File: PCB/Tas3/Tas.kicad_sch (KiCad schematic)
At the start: 36 parts, among them J1 Shelly 1, J2 Conn_01x07, J3 USB-C, Q1 PMF170XP,115, Q2 2N7002BKS, U1 MD8942, U2 Barcode, U3 CH340X

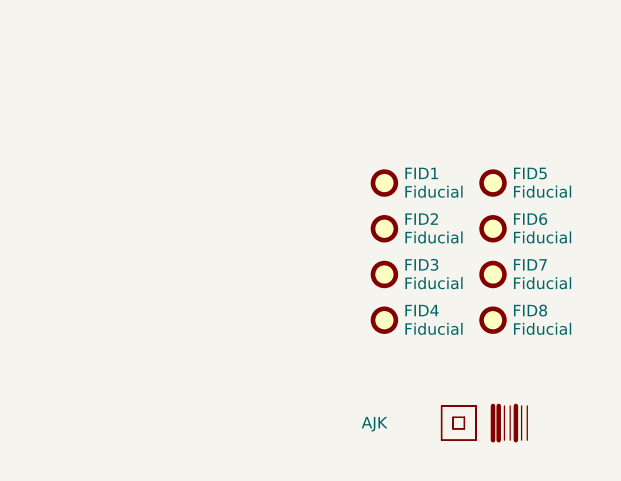
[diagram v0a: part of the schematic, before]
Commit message: Better rails
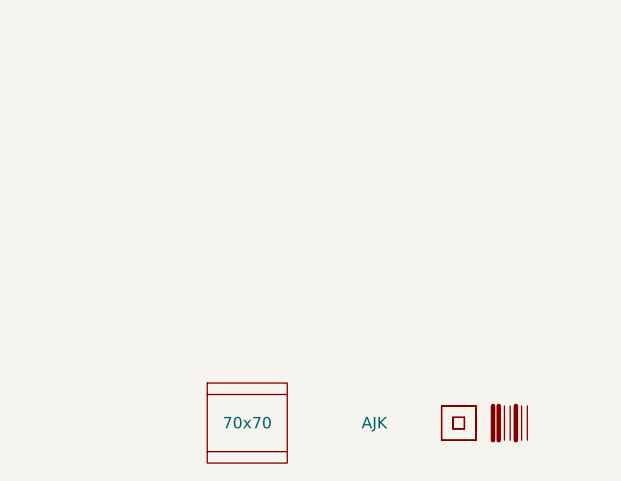
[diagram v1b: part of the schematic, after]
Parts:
- removed FID1, FID2, FID3, FID4, FID5, FID6, FID7, FID8: Fiducial, Fiducial:Fiducial_1mm_Mask2mm, symbol Mechanical:Fiducial
- added PCB1: 70x70, RevK:PCB7070, symbol RevK:PCB

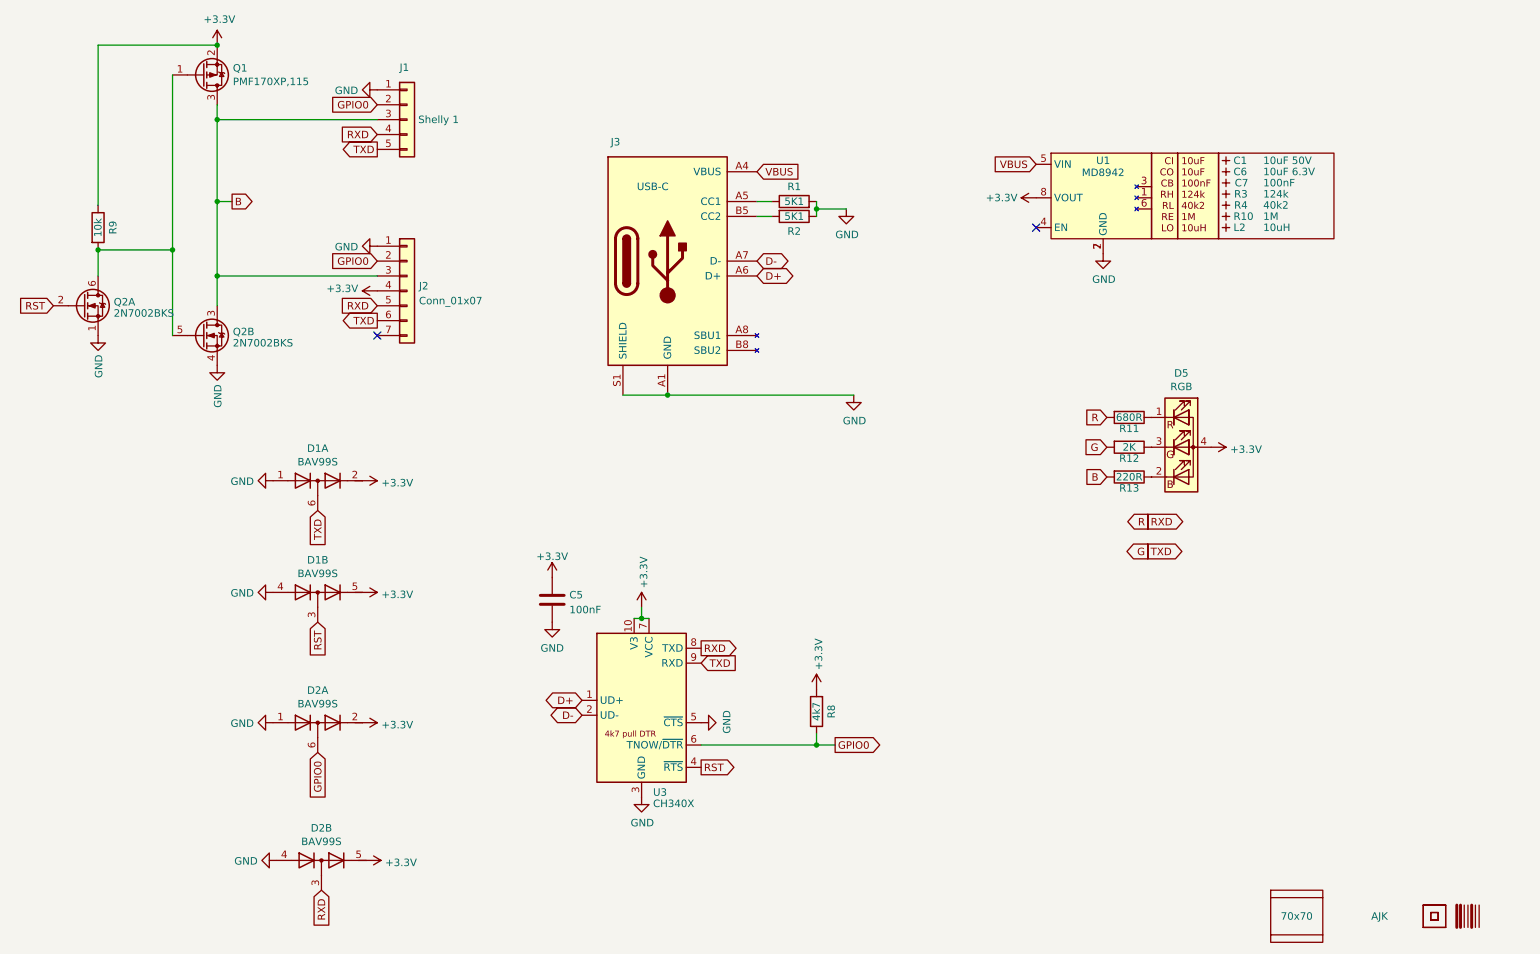
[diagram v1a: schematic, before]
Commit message: Revised totally
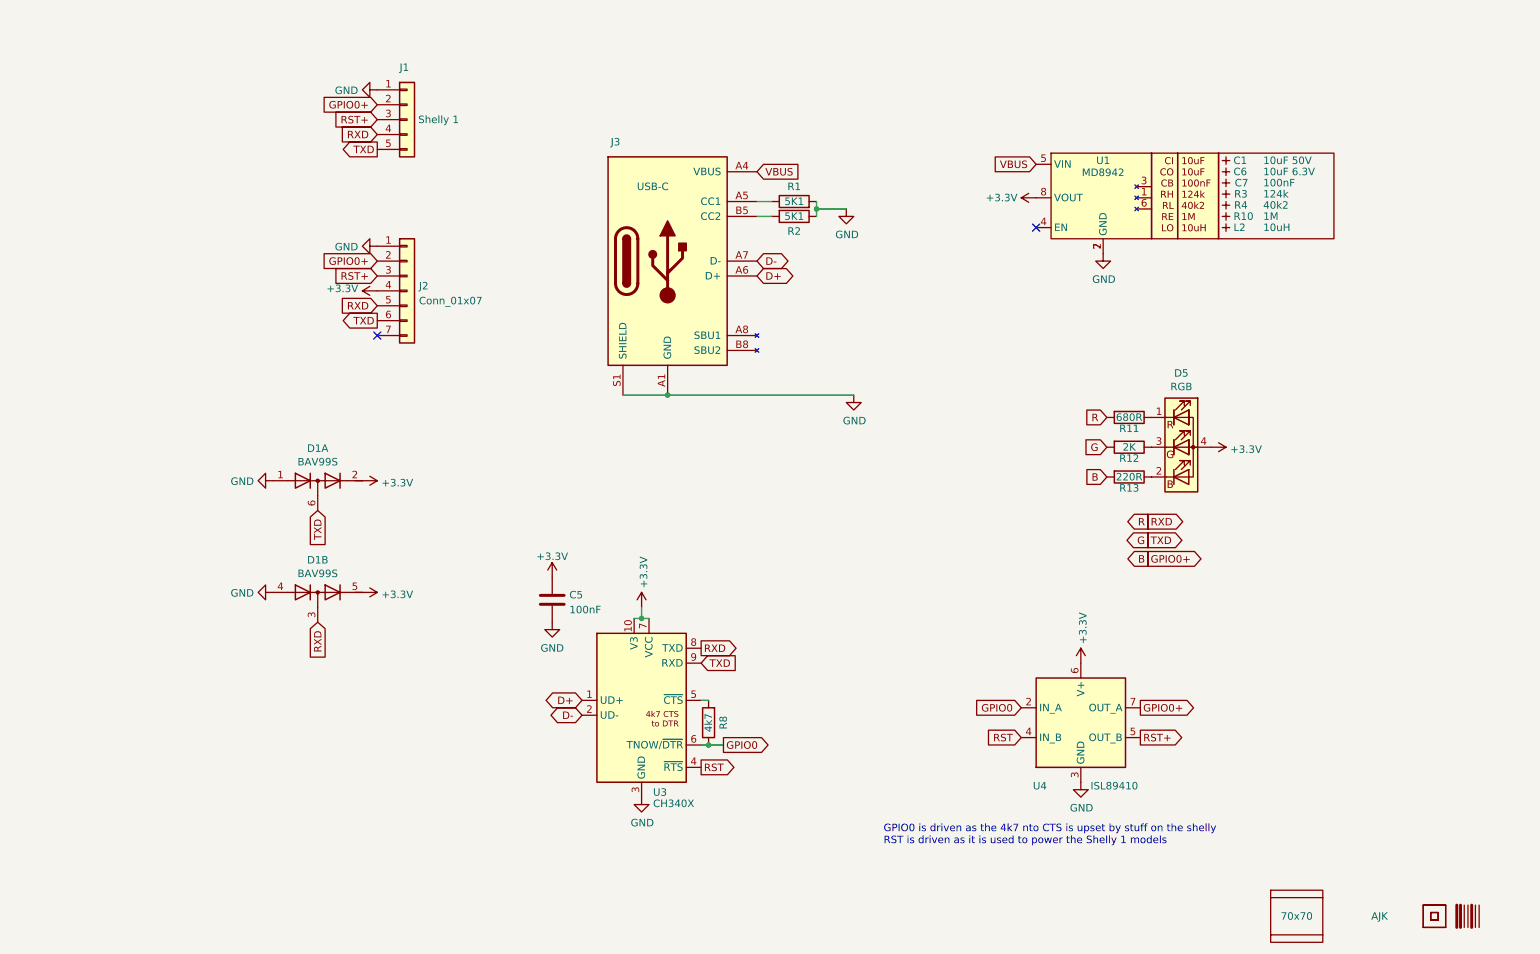
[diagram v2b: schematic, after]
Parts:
- removed D2: BAV99S, RevK:SOT-363_SC-70-6, symbol Diode:BAV99S
- removed Q1: PMF170XP,115, RevK:SOT-323_SC-70, symbol Device:Q_PMOS_GSD
- removed Q2: 2N7002BKS, RevK:SOT-363_SC-70-6, symbol Transistor_FET:FDG1024NZ
- removed R9: 10k, RevK:R_0402, symbol Device:R
- added U4: ISL89410, RevK:SO-8_3.9x4.9mm_P1.27mm, symbol Driver_FET:EL7202CN
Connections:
- net +3V3: now also U4.6 (V+); no longer R8.2
- net B: now also J1.2 (Pin_2), J2.2 (Pin_2), U4.7 (OUT_A); no longer J1.3 (Pin_3), J2.3 (Pin_3)
- net GND: now also U4.3 (GND); no longer U3.5 (~{CTS})
- net GPIO0: now also U4.2 (IN_A); no longer J1.2 (Pin_2), J2.2 (Pin_2)
- net R: now also D1.3 (K1A2)
- net RST: now also U4.4 (IN_B); no longer D1.3 (K1A2)
- new net: R8.2, U3.5 (~{CTS})
- new net RST+: J1.3 (Pin_3), J2.3 (Pin_3), U4.5 (OUT_B)
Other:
- note added: "GPIO0 is driven as the 4k7 nto CTS is upset by stuff on the shelly RST is driven as it is used to power the Shelly 1 models"
- moved on the sheet: R8

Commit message: VCUT
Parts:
- added V1, V2: ~, RevK:VCUT70, symbol RevK:VCUT
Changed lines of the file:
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@@
+    )
+  )
+  (symbol (lib_id "RevK:VCUT") (at 245.745 175.895 0) (unit 1)
+    (in_bom yes) (on_board yes) (dnp no) (fields_autoplaced)
+    (property "Reference" "V1" (at 245.745 174.625 0)
+      (effects (font (size 1.27 1.27)) hide)
+    )
+    (property "Value" "~" (at 245.745 175.895 0)
+      (effects (font (size 1.27 1.27)))
+    )
+    (property "Footprint" "RevK:VCUT70" (at 245.745 177.165 0)
+      (effects (font (size 1.27 1.27)) hide)
+    )
+    (property "Datasheet" "" (at 245.745 175.895 0)
+      (effects (font (size 1.27 1.27)) hide)
+    )
+    (instances
+      (project "Tas"
+        (path "/42713045-fffd-4b2d-ae1e-7232d705fb12"
+          (reference "V1") (unit 1)
+        )
+      )
+      (project "Reference"
+        (path "/825c70b0-4860-42b7-97dc-86bfa46e06fd"
+          (reference "V1") (unit 1)
+        )
+      )
+    )
+  )
+  (symbol (lib_id "RevK:VCUT") (at 245.745 169.545 0) (unit 1)
+    (in_bom yes) (on_board yes) (dnp no) (fields_autoplaced)
+    (property "Reference" "V2" (at 245.745 168.275 0)
+      (effects (font (size 1.27 1.27)) hide)
+    )
+    (property "Value" "~" (at 245.745 169.545 0)
+      (effects (font (size 1.27 1.27)))
+    )
+    (property "Footprint" "RevK:VCUT70" (at 245.745 170.815 0)
+      (effects (font (size 1.27 1.27)) hide)
+    )
+    (property "Datasheet" "" (at 245.745 169.545 0)
+      (effects (font (size 1.27 1.27)) hide)
+    )
+    (instances
+      (project "Tas"
+        (path "/42713045-fffd-4b2d-ae1e-7232d705fb12"
+          (reference "V2") (unit 1)
+        )
+      )
+      (project "Reference"
+        (path "/825c70b0-4860-42b7-97dc-86bfa46e06fd"
+          (reference "V1") (unit 1)
+        )
+      )
     )
   )
